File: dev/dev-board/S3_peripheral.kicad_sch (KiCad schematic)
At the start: 38 parts, among them P1 HDR-IDC-2.54-2X5P, SW5 TS342A2P, SW6 TS342A2P, SW7 TS342A2P, SW8 TS342A2P, U10 TPS2065CDBV, U11 PESD5V0U2BT, U12 PESD5V0S1BA_C5261083, U8 ZX-HY2.0-4PWZ, U9 ZX-HY2.0-4PWZ

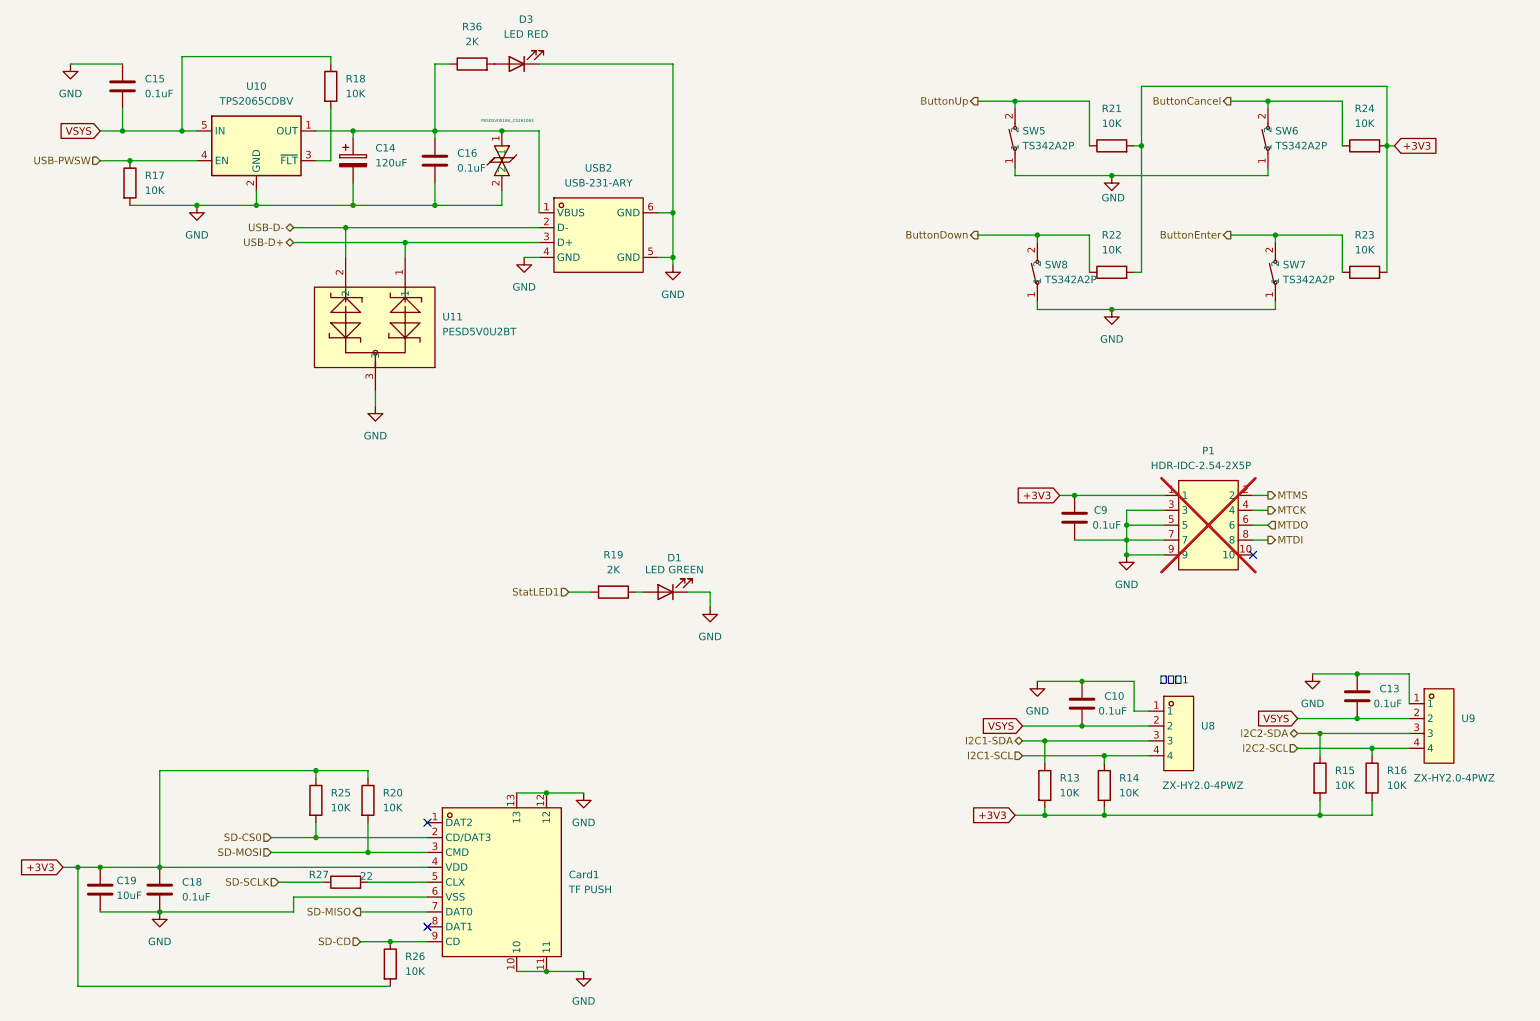
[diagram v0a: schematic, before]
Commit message: update for v3r3
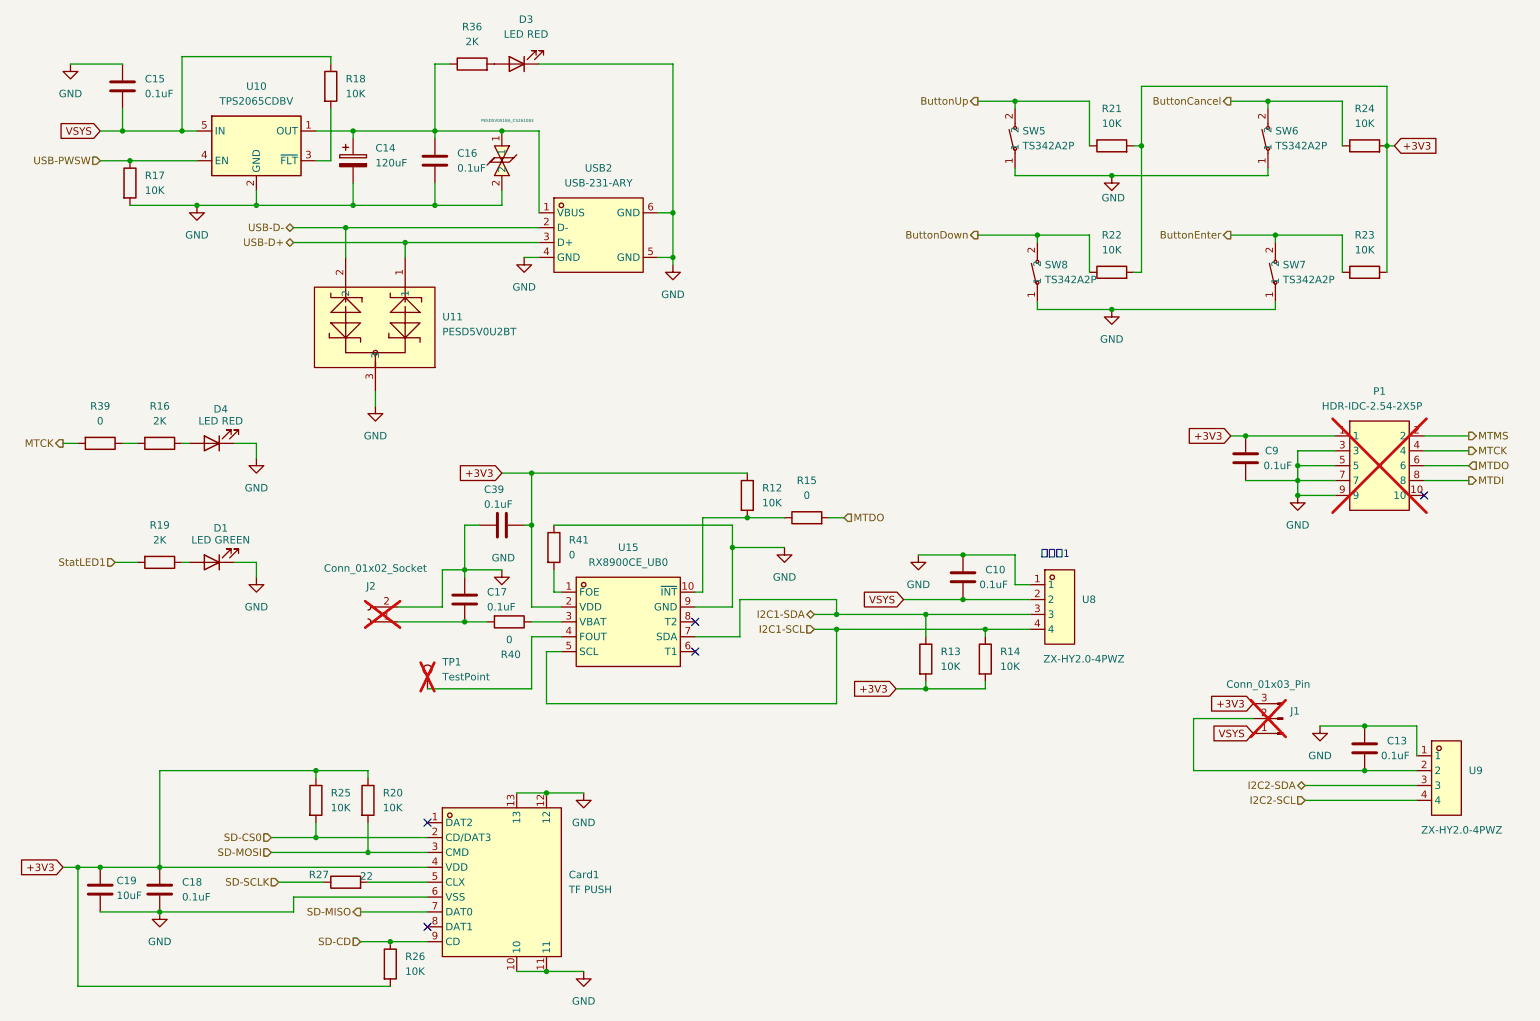
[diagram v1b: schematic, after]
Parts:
- added C17, C39: 0.1uF, Capacitor_SMD:C_0603_1608Metric, symbol Device:C
- added D4: LED RED, LED_SMD:LED_0805_2012Metric, symbol Device:LED
- added J1: Conn_01x03_Pin, Connector_PinHeader_2.54mm:PinHeader_1x03_P2.54mm_Vertical, symbol Connector:Conn_01x03_Pin
- added J2: Conn_01x02_Socket, Connector_PinSocket_2.54mm:PinSocket_1x02_P2.54mm_Vertical, symbol Connector:Conn_01x02_Socket
- added R12: 10K, Resistor_SMD:R_0603_1608Metric, symbol Device:R
- added R39, R40, R41: 0, Resistor_SMD:R_0603_1608Metric, symbol Device:R
- added TP1: TestPoint, TestPoint:TestPoint_Pad_D1.0mm, symbol Connector:TestPoint
- added U15: RX8900CE_UB0, easyeda2kicad:SMD-10_L3.2-W2.5-BL_EPSON_RX8900CE, symbol easyeda2kicad:RX8900CE_UB0
- R15: value 10K -> 0; LCSC Part C25804 -> C21189
- R16: value 10K -> 2K; LCSC Part C25804 -> C22975
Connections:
- net +3V3: now also C39.2, J1.3 (Pin_3), R12.1, U15.2 (VDD); no longer R15.2, R16.2
- net GND: now also C17.1, C39.1, D4.1 (K), J2.2 (Pin_2), R41.1, U15.9 (GND)
- net I2C1-SCL: now also U15.5 (SCL)
- net I2C1-SDA: now also U15.7 (SDA)
- net I2C2-SCL: no longer R16.1
- net I2C2-SDA: no longer R15.1
- net MTCK: now also R39.2
- net MTDO: now also R15.2
- net VSYS: now also J1.1 (Pin_1); no longer C13.2, U9.2
- new net: R16.2, R39.1
- new net: R40.1, U15.3 (VBAT)
- new net: C17.2, J2.1 (Pin_1), R40.2
- new net: R12.2, R15.1, U15.10 (~{INT})
- new net: C13.2, J1.2 (Pin_2), U9.2
- new net: D4.2 (A), R16.1
- new net: R41.2, U15.1 (FOE)
- new net: TP1.1, U15.4 (FOUT)
- no-connect marks 3 -> 5
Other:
- moved on the sheet: C10, C13, C9, D1, P1, R13, R14, R19, U8, U9

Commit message: v3 dev r3 candidate2
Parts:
- D4: footprint LED_SMD:LED_0805_2012Metric -> LED_SMD:LED_0603_1608Metric; LCSC Part C2297 -> C2286
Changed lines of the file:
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@@
 			)
 		)
-		(property "Footprint" "LED_SMD:LED_0805_2012Metric"
+		(property "Footprint" "LED_SMD:LED_0603_1608Metric"
 			(at 53.34 87.63 0)
 			(effects
@@
 			)
 		)
-		(property "LCSC Part" "C2297"
+		(property "LCSC Part" "C2286"
 			(at 53.34 87.63 0)
 			(effects
